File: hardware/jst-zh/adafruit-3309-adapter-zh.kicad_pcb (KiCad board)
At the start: 2 copper layers, 20.3 x 33 mm, 3 parts, among them J1 S6B-ZR-SM4A-TF(LF)(SN), J2 Conn_01x08_Female, J3 Conn_01x08_Female

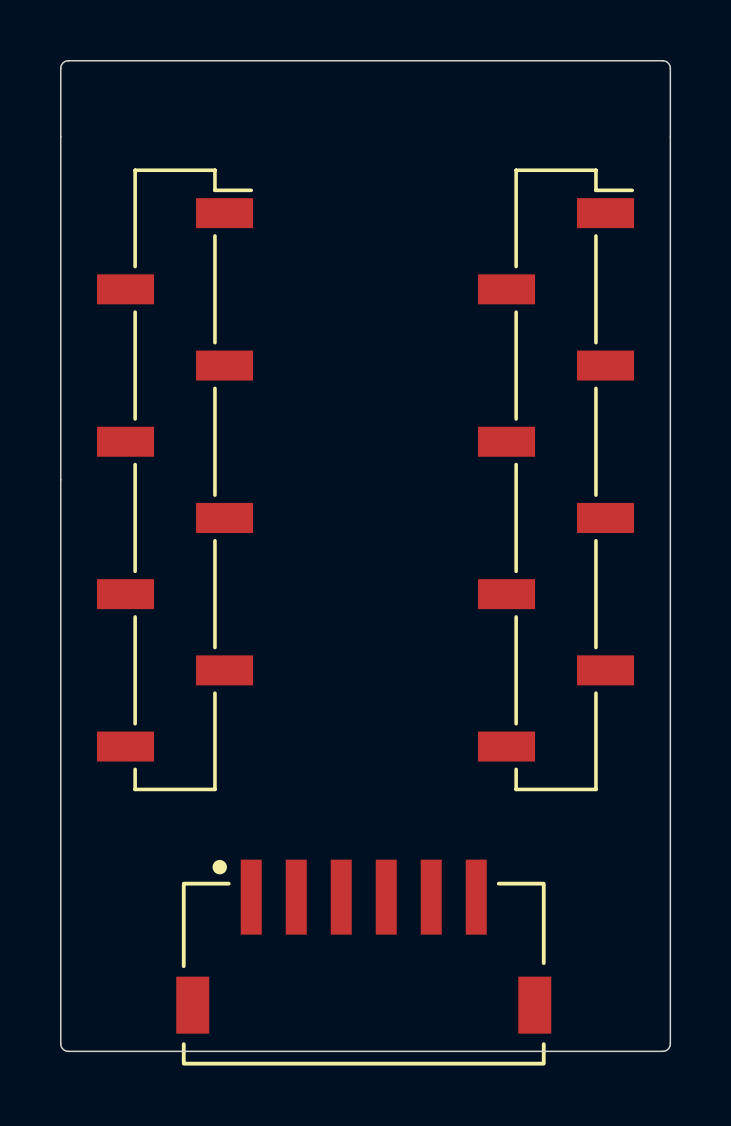
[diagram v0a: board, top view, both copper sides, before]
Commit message: Routing done
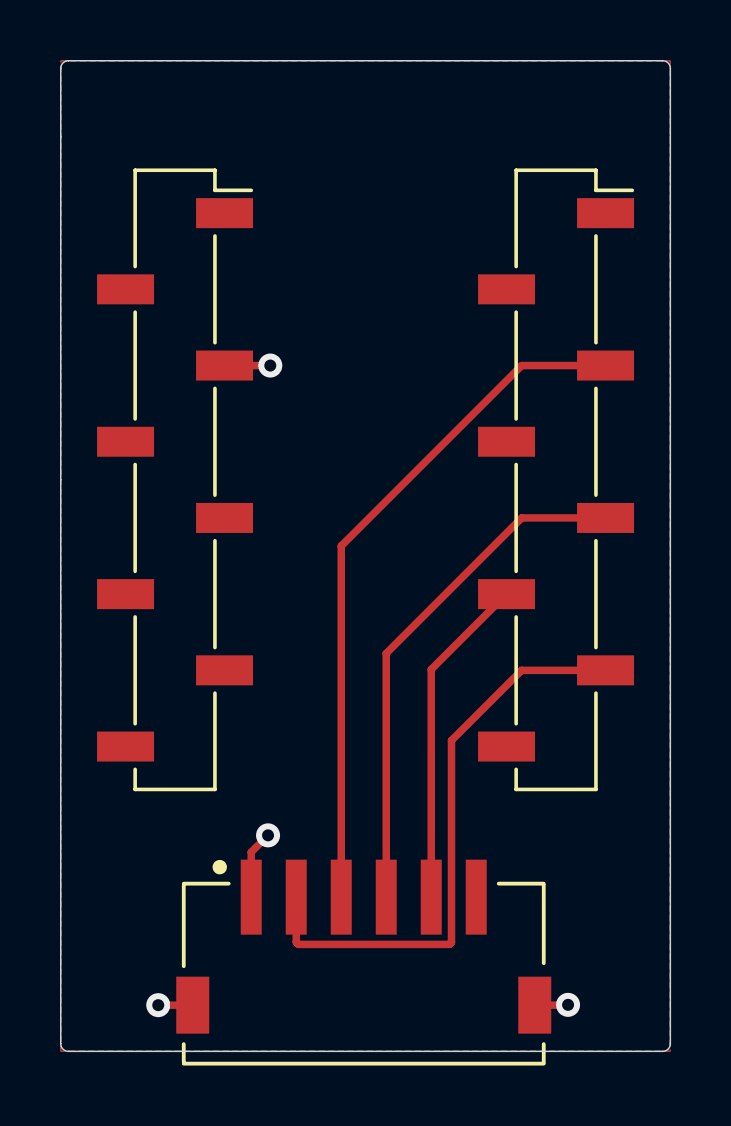
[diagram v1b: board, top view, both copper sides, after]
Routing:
- net /DTR: track 0.00 -> 23.0 mm
- net /RTS: track 0.00 -> 19.6 mm
- net /TX: track 0.00 -> 17.3 mm
- net /RX: track 0.00 -> 11.1 mm
- net GND: track 0.00 -> 6.08 mm, vias 0 -> 4
- added copper zone on F.Cu, net +5V
- added copper zone on B.Cu, net GND
